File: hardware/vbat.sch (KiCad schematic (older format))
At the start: 5 parts

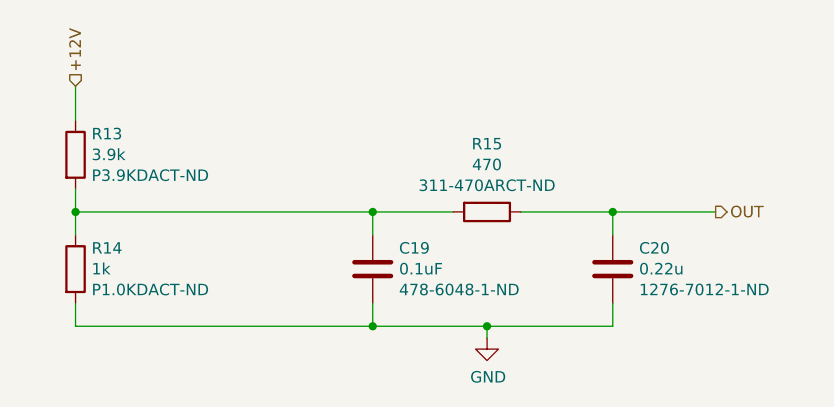
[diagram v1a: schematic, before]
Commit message: hardware rev2 - layout complete
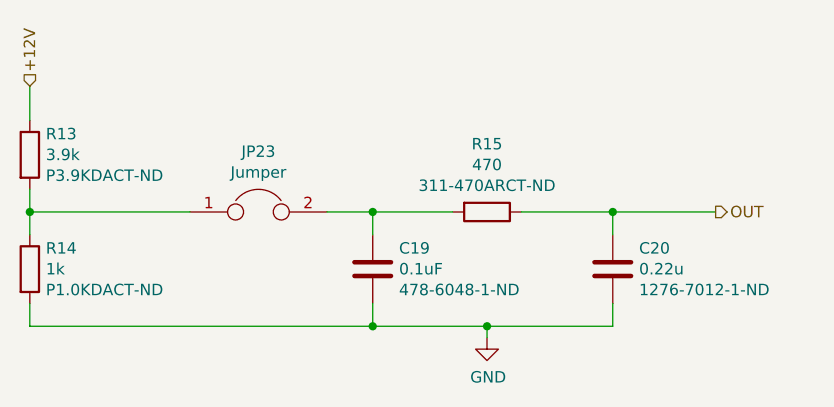
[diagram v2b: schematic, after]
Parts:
- added JP23: Jumper, Pin_Headers:Pin_Header_Straight_1x02_Pitch2.54mm, symbol Device:Jumper
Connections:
- net at R13.2, R14.1: now also JP23.1; no longer C19.1, R15.2
- new net: C19.1, JP23.2, R15.2
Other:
- moved on the sheet: R13, R14
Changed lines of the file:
@@
 L Device:R R13
 U 1 1 5C66139D
-P 3150 4100
-F 0 "R13" H 3220 4191 50  0000 L CNN
-F 1 "3.9k" H 3220 4100 50  0000 L CNN
-F 2 "Resistors_SMD:R_0805_HandSoldering" V 3080 4100 50  0001 C CNN
-F 3 "~" H 3150 4100 50  0001 C CNN
-F 4 "P3.9KDACT-ND" H 3220 4009 50  0000 L CNN "DIGIKEY"
-	1    3150 4100
+P 2950 4100
+F 0 "R13" H 3020 4191 50  0000 L CNN
+F 1 "3.9k" H 3020 4100 50  0000 L CNN
+F 2 "Resistors_SMD:R_0805_HandSoldering" V 2880 4100 50  0001 C CNN
+F 3 "~" H 2950 4100 50  0001 C CNN
+F 4 "P3.9KDACT-ND" H 3020 4009 50  0000 L CNN "DIGIKEY"
+	1    2950 4100
 	1    0    0    -1
 $EndComp
@@
 L Device:R R14
 U 1 1 5C6613E7
-P 3150 4600
-F 0 "R14" H 3220 4691 50  0000 L CNN
-F 1 "1k" H 3220 4600 50  0000 L CNN
-F 2 "Resistors_SMD:R_0805_HandSoldering" V 3080 4600 50  0001 C CNN
-F 3 "~" H 3150 4600 50  0001 C CNN
-F 4 "P1.0KDACT-ND" H 3220 4509 50  0000 L CNN "DIGIKEY"
-	1    3150 4600
+P 2950 4600
+F 0 "R14" H 3020 4691 50  0000 L CNN
+F 1 "1k" H 3020 4600 50  0000 L CNN
+F 2 "Resistors_SMD:R_0805_HandSoldering" V 2880 4600 50  0001 C CNN
+F 3 "~" H 2950 4600 50  0001 C CNN
+F 4 "P1.0KDACT-ND" H 3020 4509 50  0000 L CNN "DIGIKEY"
+	1    2950 4600
 	1    0    0    -1
 $EndComp
@@
 	4800 4350 4450 4350
 Wire Wire Line
-	3150 4350 3150 4250
+	2950 4350 2950 4250
 Wire Wire Line
-	3150 4450 3150 4350
-Connection ~ 3150 4350
+	2950 4450 2950 4350
+Connection ~ 2950 4350
 Wire Wire Line
 	4450 4450 4450 4350
-Connection ~ 4450 4350
 Wire Wire Line
-	4450 4350 3150 4350
+	3650 4350 2950 4350
 Wire Wire Line
-	3150 3950 3150 3800
+	2950 3950 2950 3800
 Wire Wire Line
 	5500 4750 5500 4850
@@
 	4950 4850 4950 4900
 Wire Wire Line
-	3150 4750 3150 4850
-Wire Wire Line
-	3150 4850 4450 4850
+	2950 4750 2950 4850
 Connection ~ 4950 4850
 Wire Wire Line
 	4450 4750 4450 4850
-Connection ~ 4450 4850
 Wire Wire Line
 	4450 4850 4950 4850
@@
 	1    0    0    -1
 $EndComp
-Text HLabel 3150 3800 1    50   Input ~ 0
+Text HLabel 2950 3800 1    50   Input ~ 0
 +12V
+$Comp
+L Device:Jumper JP?
+U 1 1 5D014F1D
+P 3950 4350
+AR Path="/5D014F1D" Ref="JP?"  Part="1"
+AR Path="/5C661325/5D014F1D" Ref="JP23"  Part="1"
+F 0 "JP23" H 3950 4614 50  0000 C CNN
+F 1 "Jumper" H 3950 4523 50  0000 C CNN
+F 2 "Pin_Headers:Pin_Header_Straight_1x02_Pitch2.54mm" H 3950 4350 50  0001 C CNN
+F 3 "~" H 3950 4350 50  0001 C CNN
+	1    3950 4350
+	1    0    0    -1
+$EndComp
+Wire Wire Line
+	4250 4350 4450 4350
+Connection ~ 4450 4350
+Wire Wire Line
+	2950 4850 4450 4850
+Connection ~ 4450 4850
 $EndSCHEMATC
